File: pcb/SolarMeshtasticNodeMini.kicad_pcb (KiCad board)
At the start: 4 copper layers, 71.3 x 92.8 mm, 42 parts, among them J1 Conn_01x02_Socket, J2 Conn_01x02_Socket, J3 Conn_01x04_Socket, J4 Conn_01x03_Pin, J5 Conn_01x04_Socket, J6 Conn_01x03_Pin, J7 Conn_01x04_Socket, Q1 MMBT2222A, Q2 MMBT2222A, U1 BQ25185, U2 HT-CT62, U3 HE9073A30MR, U4 APX803L05-32SA-7, U9 SS26_C5350986

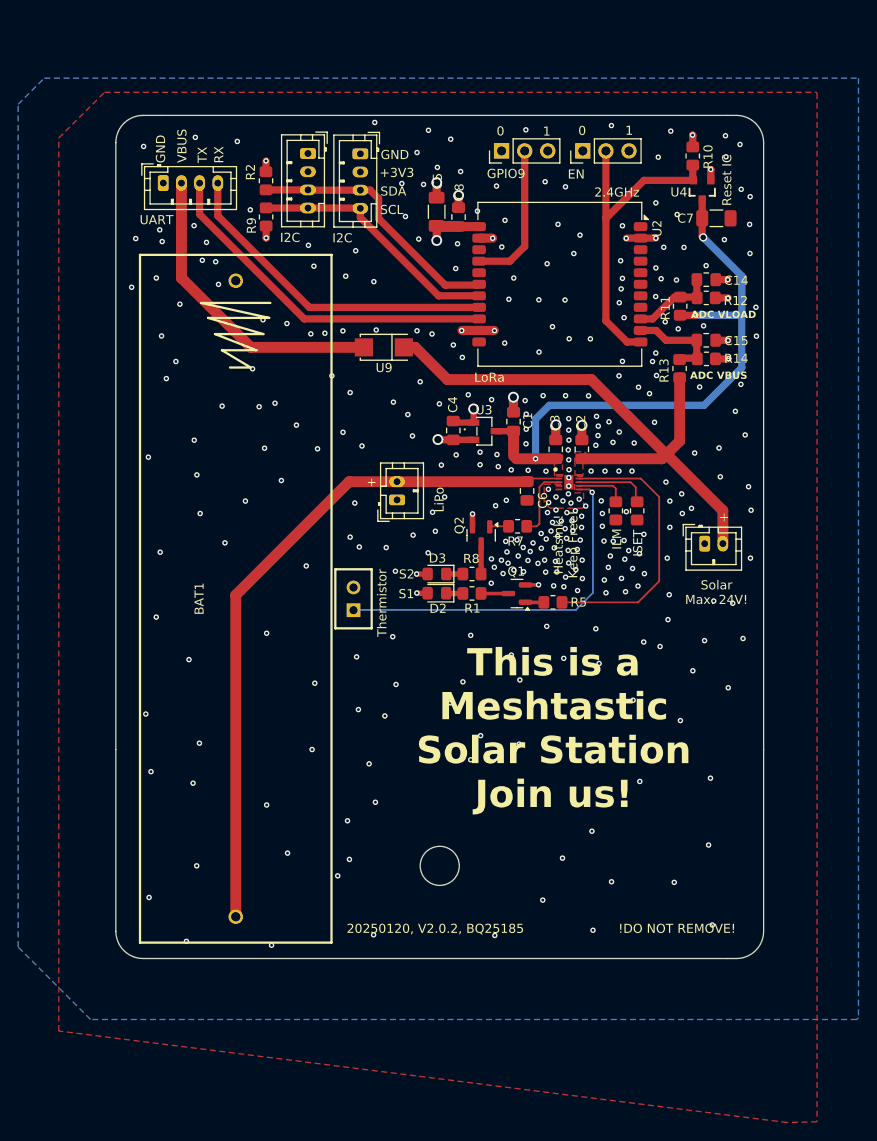
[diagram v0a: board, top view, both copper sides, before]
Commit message: pcb, sch: first layout done
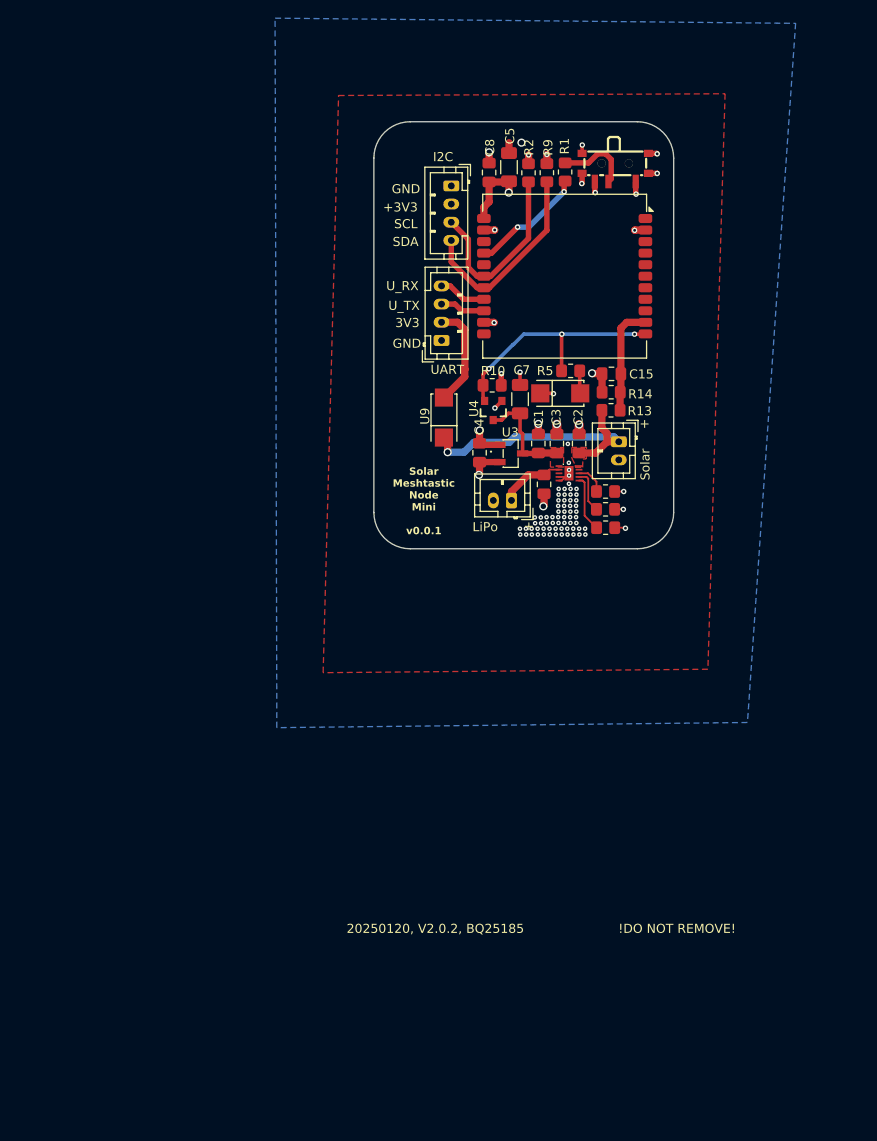
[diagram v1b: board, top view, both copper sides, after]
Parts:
- removed BAT1: BH-26650-A5BJ001, footprints:BAT-TH_BH-18650-A1AJ005
- removed C14: 100nF, Capacitor_SMD:C_0805_2012Metric_Pad1.18x1.45mm_HandSolder
- removed D2, D3: LED, LED_SMD:LED_0805_2012Metric_Pad1.15x1.40mm_HandSolder
- removed H3: MountingHole, MountingHole:MountingHole_4.3mm_M4_DIN965
- removed J1: Conn_01x02_Socket, Connector_JST:JST_PH_B2B-PH-K_1x02_P2.00mm_Vertical
- removed J6: Conn_01x03_Pin, Connector_PinHeader_2.54mm:PinHeader_1x03_P2.54mm_Vertical
- removed J7: Conn_01x04_Socket, Connector_JST:JST_PH_B4B-PH-K_1x04_P2.00mm_Vertical
- removed Q1, Q2: MMBT2222A, Package_TO_SOT_SMD:SOT-23
- removed R11, R12: 1M, Resistor_SMD:R_0805_2012Metric_Pad1.20x1.40mm_HandSolder
- removed R7: 10k, Resistor_SMD:R_0805_2012Metric_Pad1.20x1.40mm_HandSolder
- removed R8: 1k, Resistor_SMD:R_0805_2012Metric_Pad1.20x1.40mm_HandSolder
- added SW1: SSSS811101, footprints:SW-SMD_SSSS811101, F.Cu at (238.1, 35.0)
- added SW2: SW_Push, footprints:SMA_L4.3-W2.6-LS5.1-RD, F.Cu at (232.0, 59.9)
- C7: value 22uF -> 1uF
- J4: value Conn_01x03_Pin -> Conn_01x02_Pin; footprint Connector_PinHeader_2.54mm:PinHeader_1x03_P2.54mm_Vertical -> Connector_JST:JST_PH_B2B-PH-K_1x02_P2.00mm_Vertical
- R1: value 1k -> R
- R5: value 10k -> 470
- R6: footprint footprints:RES-TH_L6.5-W4.0-P2.50-D0.5 -> Resistor_SMD:R_0805_2012Metric_Pad1.20x1.40mm_HandSolder
- moved R1 47.5 mm to (232.6, 35.5), turned to -90 degrees
- moved J4 38.5 mm to (226.7, 71.7), turned to 180 degrees
- moved J3 35.2 mm to (218.9, 54.1), turned to 90 degrees
- moved R10 33.5 mm to (224.5, 59.0), turned to 180 degrees
- moved U4 33.4 mm to (224.6, 61.7)
- moved R9 31.3 mm to (230.5, 35.6), turned to 90 degrees
- moved C7 29.4 mm to (227.6, 60.5), turned to -90 degrees
- moved R2 28.9 mm to (228.5, 35.6)
- moved R6 28.8 mm to (237.0, 74.7), turned to 0 degrees
- moved R5 25.6 mm to (233.2, 57.4), turned to 180 degrees
- moved J5 16.2 mm to (220.0, 37.1)
- moved J2 14.7 mm to (238.5, 65.2), turned to -90 degrees
- moved R14 11.1 mm to (237.6, 59.8), turned to 180 degrees
- moved C15 11.1 mm to (237.7, 57.8), turned to 180 degrees
- moved U9 10.2 mm to (219.2, 62.6), turned to 90 degrees
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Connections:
- J2 pad 1: GND -> /VBUS
- J2 pad 2: /VBUS -> GND
- J4 pad 1: GND -> /VLIPO
- J4 pad 2: /ESP32_BOOTLOADER_MODE_1 -> GND
- R1 pad 2: Net-(Q1-C) -> /ESP32_BOOTLOADER_MODE_1
- R5 pad 2: /LED_STAT1 -> /ESP32_ENABLE
- U1 pad 3: /LED_STAT2 -> unconnected-(U1-STAT2-Pad3)
- U1 pad 9: /LED_STAT1 -> unconnected-(U1-STAT1-Pad9)
- U2 pad 9: /ADC_LIPO -> unconnected-(U2-GPIO1-Pad9)
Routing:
- net /VLIPO: track 75.8 -> 7.20 mm
- net /VLOAD: track 66.0 -> 11.6 mm, vias 3 -> 0
- net /VBUS: track 64.7 -> 30.4 mm, vias 0 -> 1
- net Net-(U1-TS/MR): track 40.3 -> 6.23 mm, vias 1 -> 0
- net /U_TX: track 39.0 -> 4.97 mm
- net /U_RX: track 36.5 -> 5.28 mm
- net /LED_STAT1: track 30.6 -> 0.00 mm
- net Net-(J3-Pin_2): track 33.7 -> 11.3 mm
- net /ESP32_ENABLE: track 36.6 -> 26.9 mm, vias 0 -> 3
- net /ADC_LIPO: track 9.10 -> 0.00 mm
- net /I2C_SCL: track 28.9 -> 20.7 mm
- net /LED_STAT2: track 7.92 -> 0.00 mm
- net Net-(R1-Pad1): track 1.81 -> 8.30 mm
- net /I2C_SDA: track 28.0 -> 22.0 mm
- net Net-(U1-ISET): track 8.09 -> 3.76 mm
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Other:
- board size 71.3 x 92.8 mm -> 33 x 47 mm
- rule pad_to_mask_clearance: 0.05 -> 0
- board text added: "3V3"
- board text added: "Solar"
- board text added: "Solar Meshtastic Node Mini v0.0.1"
- board text added: "U_RX"
- board text added: "U_TX"
- board text removed: "0"
- board text removed: "1"
- board text removed: "2.4GHz"
- board text removed: "ADC VBUS"
- board text removed: "ADC VLOAD"
- board text removed: "EN"
- board text removed: "GPIO9"
- board text removed: "Heatsink! Keep Free!"
- board text removed: "ILM"
- board text removed: "ISET"
- board text removed: "LoRa"
- board text removed: "RX"
- board text removed: "Reset IC"
- board text removed: "S1"
- board text removed: "S2"
- board text removed: "Solar Max. 24V!"
- board text removed: "TX"
- board text removed: "Thermistor"
- board text removed: "This is a Meshtastic Solar Station Join us!"
- board text removed: "VBUS"
